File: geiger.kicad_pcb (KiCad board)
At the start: 2 copper layers, 117.6 x 73.2 mm, 37 parts, among them SW1 SW_SPST, T1 IRFP450, T2 P55NF06, T3 BC517, U1 NE555P, U2 LM336Z25, U3 LM311, U4 STEP-DOWN-5V, U5 nodemcu-esp32, U6 GEIGERTUBE-STS6

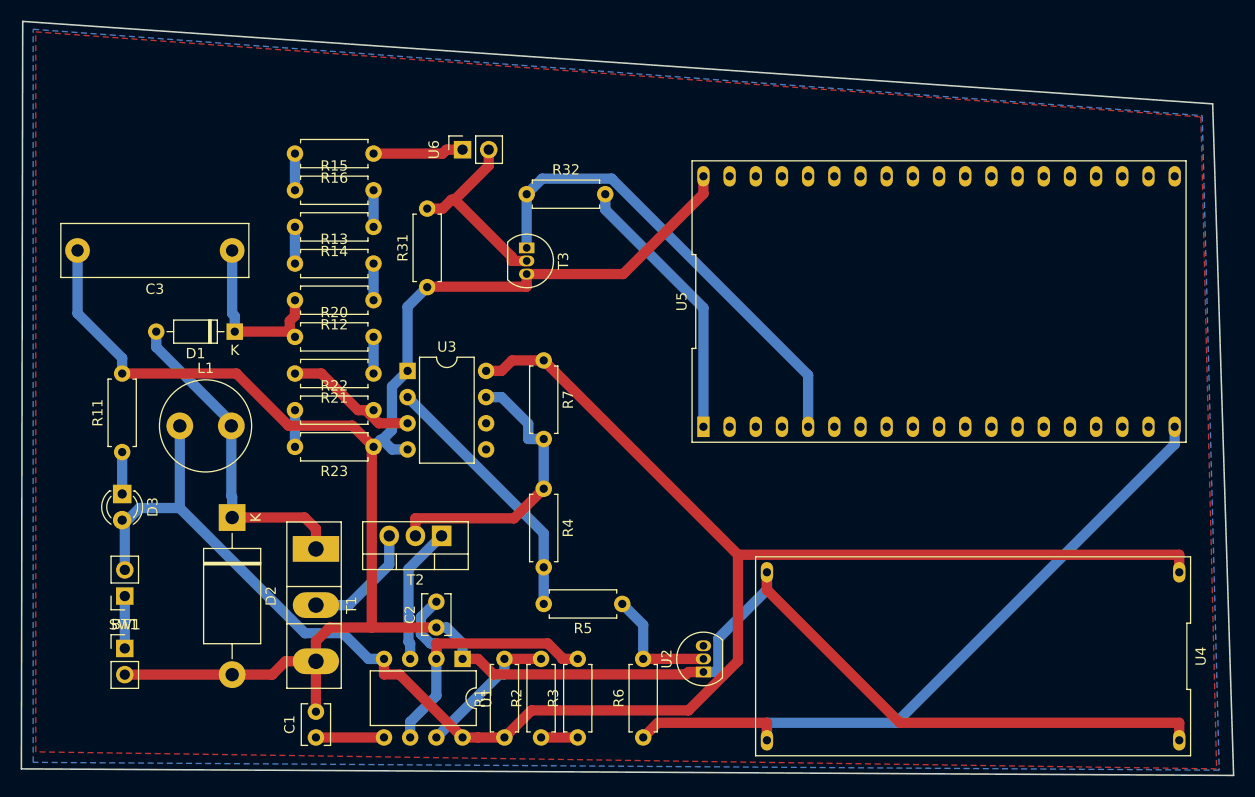
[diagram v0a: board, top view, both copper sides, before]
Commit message: a
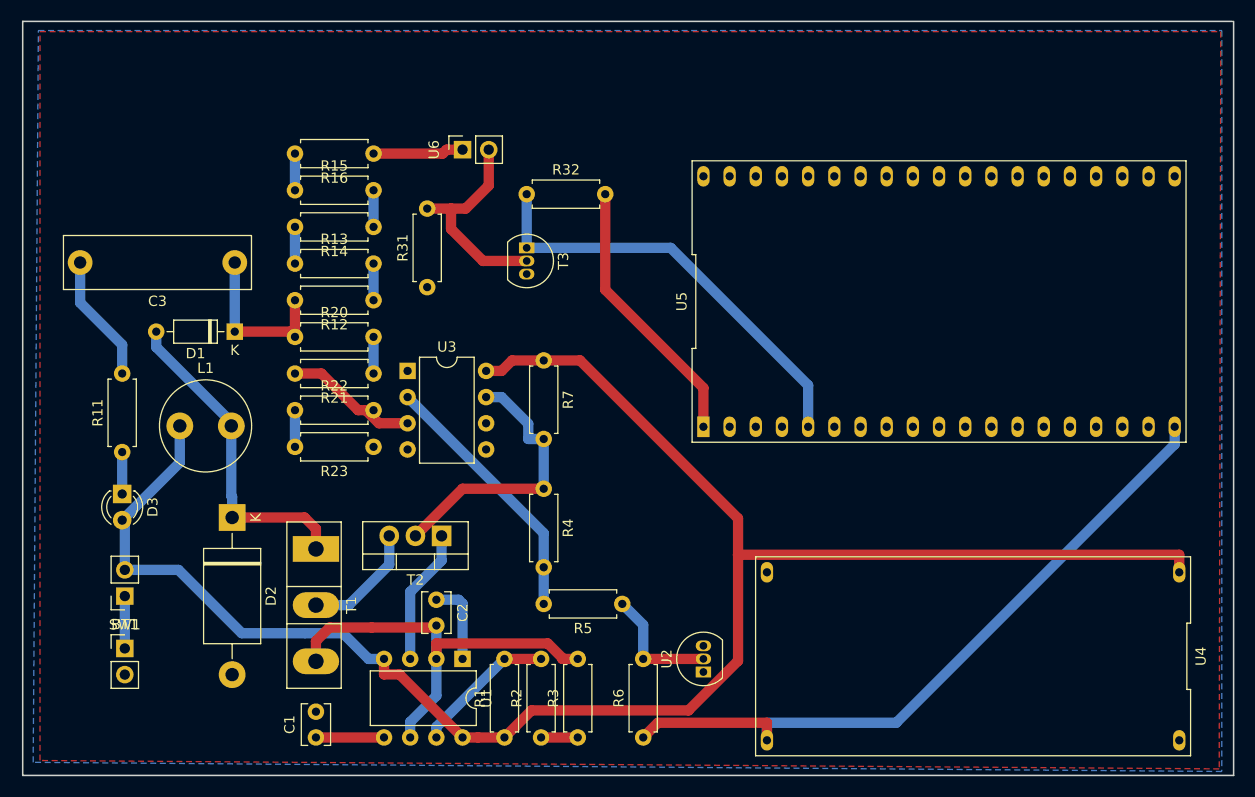
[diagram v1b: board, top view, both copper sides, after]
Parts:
- moved C2 2.69 mm to (57.9, 180.7), turned to 270 degrees
- moved C3 1.20 mm to (38.4, 148.0)
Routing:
- net GND: track 240.9 -> 35.1 mm
- net Net-(C2-Pad2): track 31.7 -> 27.8 mm
- net Net-(R32-Pad1): track 46.0 -> 42.3 mm
- net +8V: track 173.6 -> 176.1 mm
- net Net-(R31-Pad2): track 18.9 -> 21.0 mm
- net Net-(R4-Pad1): track 28.3 -> 27.3 mm
- net Net-(C3-Pad1): track 17.3 -> 16.3 mm
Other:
- board size 117.6 x 73.2 mm -> 117.5 x 73.2 mm
- net class AAA added: clearance 0.2, trace_width 1, via_dia 0.8, via_drill 0.4
